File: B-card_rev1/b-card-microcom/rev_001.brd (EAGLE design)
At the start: 160 x 100 mm, 43 parts, among them IC1 DMN2041L-7, IC2 DMN2041L-7, IC3 DMN2041L-7, J1 10118192-0002LF, J2 S2B-PH-SM4-TB(LF)(SN), SW1 B3AL-1000P, U1 ATMEGA32U4-MU, U2 MCP73832T-5ACI, U3 TPS61097-33, Y1 CSTNE8M00GH5C000R0

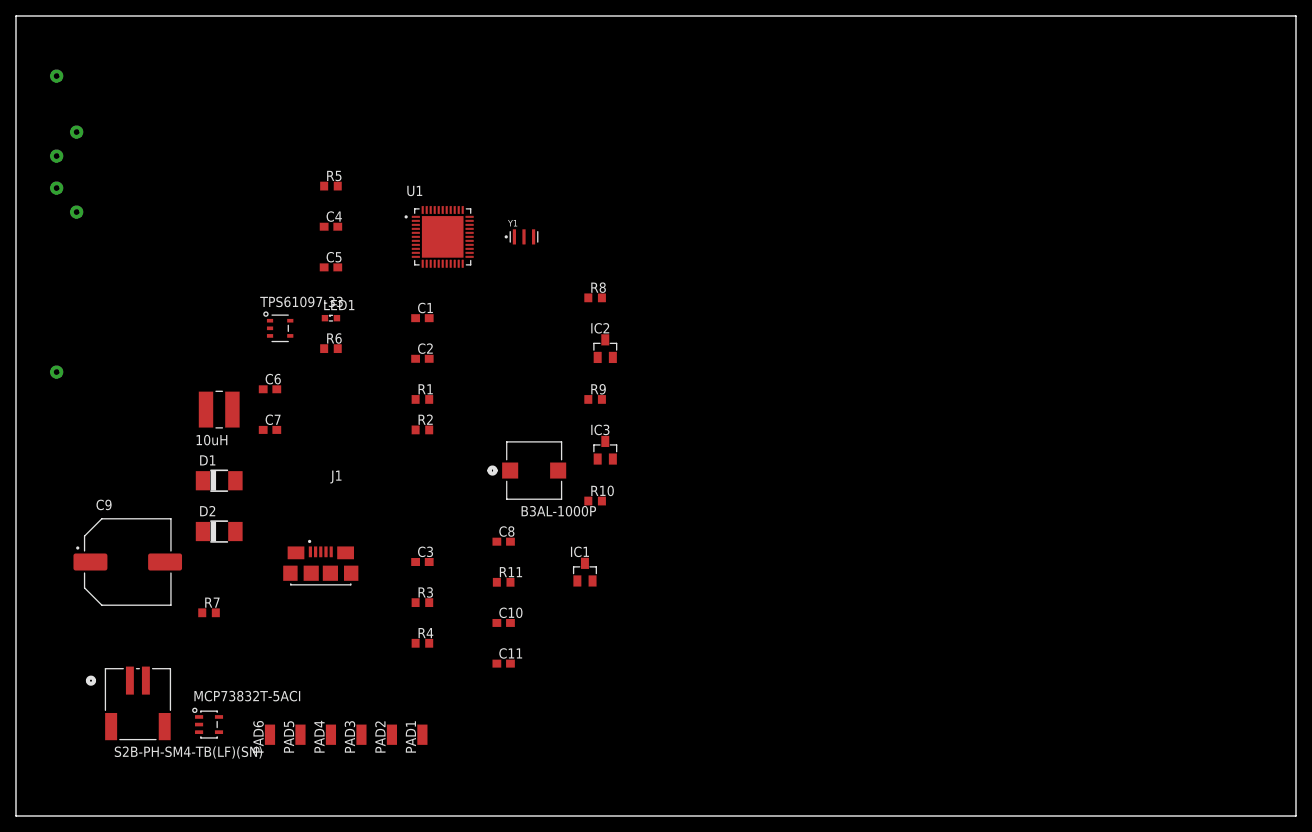
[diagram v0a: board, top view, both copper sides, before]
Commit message: update
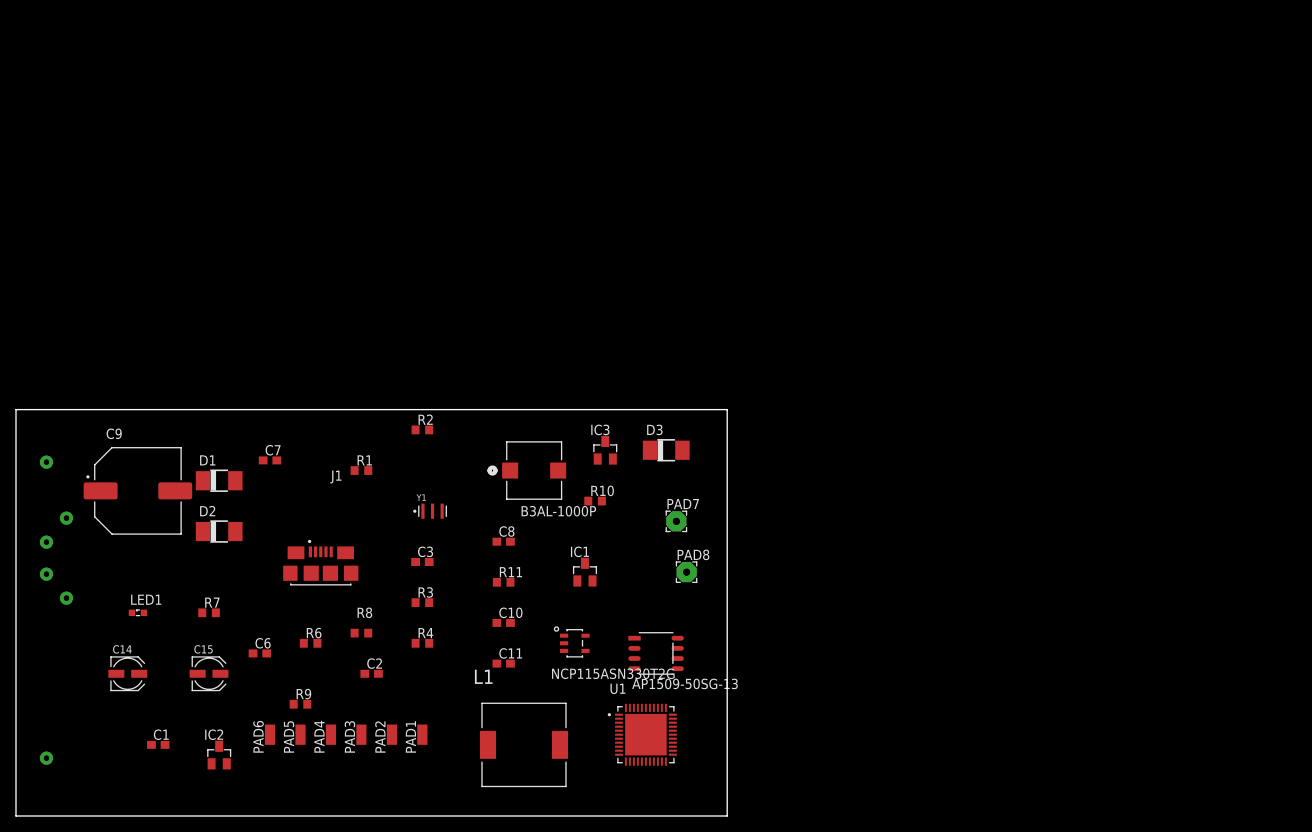
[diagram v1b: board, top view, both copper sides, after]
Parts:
- removed C4, C5: 4.7uF, rcl:C0603
- removed J2: S2B-PH-SM4-TB(LF)(SN), ul_S2B-PH-SM4-TB-LF-SN:CONN_S2B-PH-SM4-TB_JST
- removed R5: 2k, rcl:R0603
- removed U3: TPS61097-33, ul_TPS61097-33DBVR:DBV5-L
- added C14, C15: 470uf, rcl:UD-4X5,8_NICHICON
- added D3: CDBA340-HF, diode:DO-214AC
- added PAD7, PAD8: WIREPAD2,54/0,9, wirepad:2,54/0,9
- added U4: NCP115ASN330T2G, ul_NCP115ASN330T2G:TSOP-5-483-N_ONS
- L1: value 10uH -> 47uh; device ul_SDR0403-100ML:IND_BOURNS_SDR0403 -> Wuerth Elektronik - 7447714470:WUERTH_ELEKTRONIK_7447714470_0
- U2: value MCP73832T-5ACI -> AP1509-50SG-13; device ul_MCP73832T-5ACI-OT:SOT-23-5_MC_MCH-L -> ul_AP1509-50SG-13:SOP-8L_DIO
- moved IC2 70.1 mm to (25.4, 7.62)
- moved U1 67.2 mm to (78.7, 10.2)
- moved C1 62.7 mm to (17.8, 8.89)
- moved L1 56.6 mm to (63.5, 8.89)
- moved U2 56.6 mm to (80.0, 20.3)
- moved R9 53.0 mm to (35.6, 14.0)
- moved R8 51.1 mm to (43.2, 22.9)
- moved NICR1 48.3 mm to (3.81, 30.5)
- moved LED1 44.0 mm to (15.2, 25.4)
- moved C2 39.9 mm to (44.5, 17.8)
- moved R6 36.9 mm to (36.8, 21.6)
- moved Y1 36.1 mm to (52.1, 38.1)
- moved C6 33.0 mm to (30.5, 20.3)
- moved R1 11.7 mm to (43.2, 43.2)
- moved C9 8.98 mm to (15.2, 40.6)
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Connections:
- removed net +4.1V: C4.1, D2.A, IC1.D, IC2.D, IC3.D, J2.1, U2.3
- removed net N$5: R5.2, U2.5
- removed net N$8: L1.1, U3.5
- new net +8V: C14.+, PAD7.1, U2.1
- net +3V3: now also LED1.A, U4.5; no longer U3.4
- net +5V: now also C15.+, D2.A, IC1.D, IC2.D, IC3.D, L1.2, U2.3; no longer C5.1, LED1.A, U2.4
- net GND: now also C14.-, C15.-, D3.A, PAD8.1, R6.1, U2.4, U2.5, U2.6, U2.7, U2.8, U4.2; no longer C4.2, C5.2, J2.2, R5.1, U2.2, U3.2
- net N$10: now also U4.1, U4.3; no longer L1.2, U3.1, U3.3
- net N$7: now also D3.C, L1.1, U2.2; no longer R6.1, U2.1
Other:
- board size 160 x 100 mm -> 88.9 x 50.8 mm
